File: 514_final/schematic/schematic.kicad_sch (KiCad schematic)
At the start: 21 parts, among them M1 Stepper_Motor_unipolar_5pin, SW1 SW_Push, SW2 SW_Push, U1 ULN2003

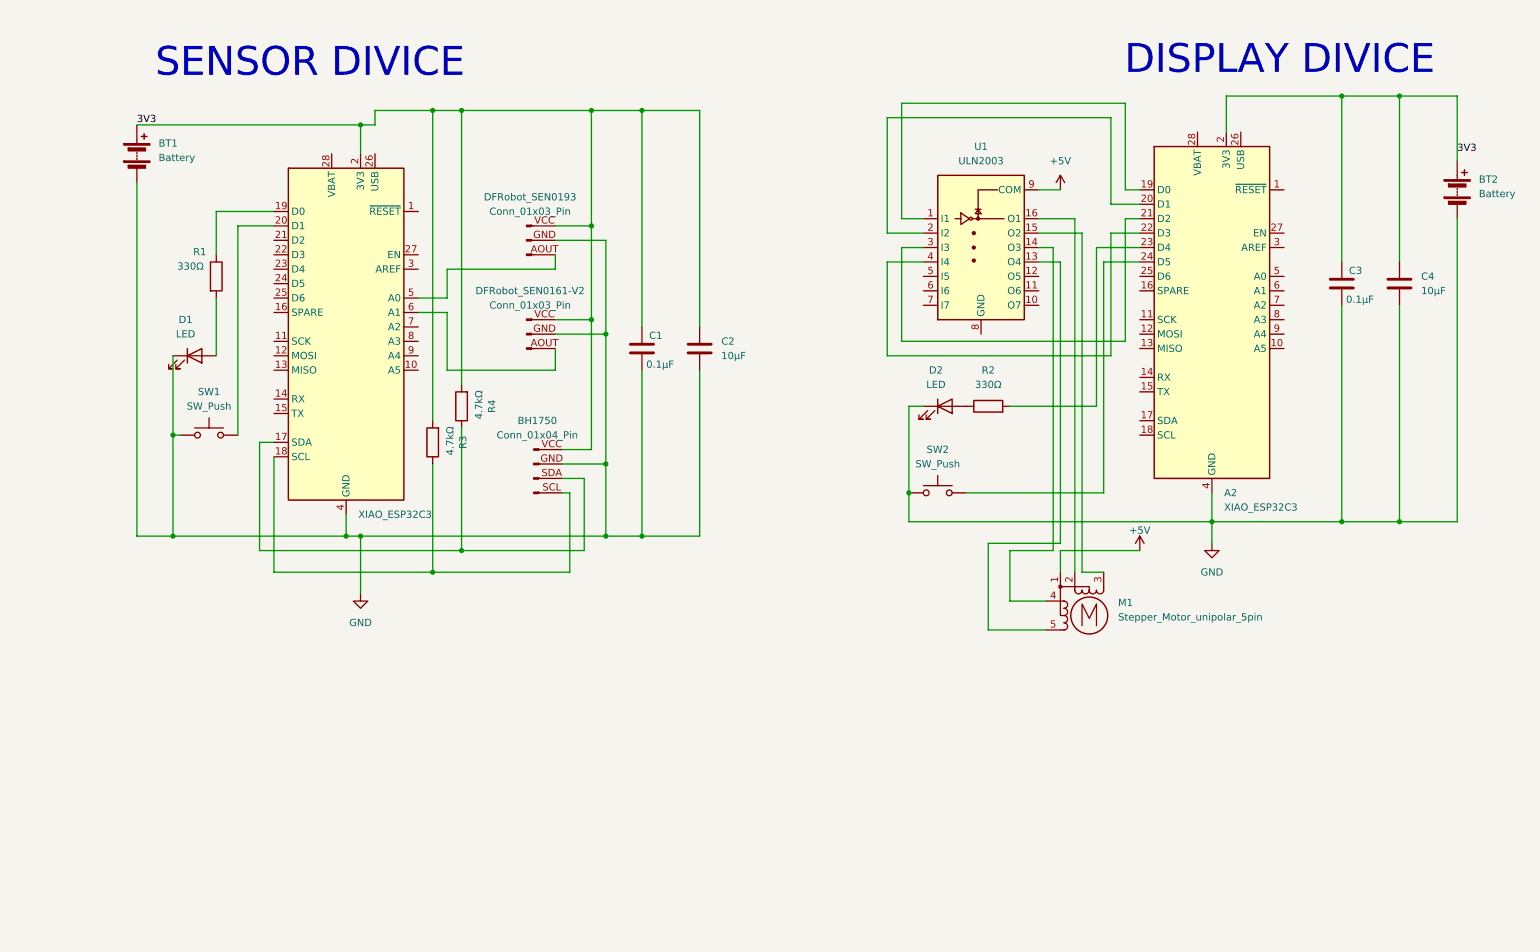
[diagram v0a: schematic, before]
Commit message: PCB 0203
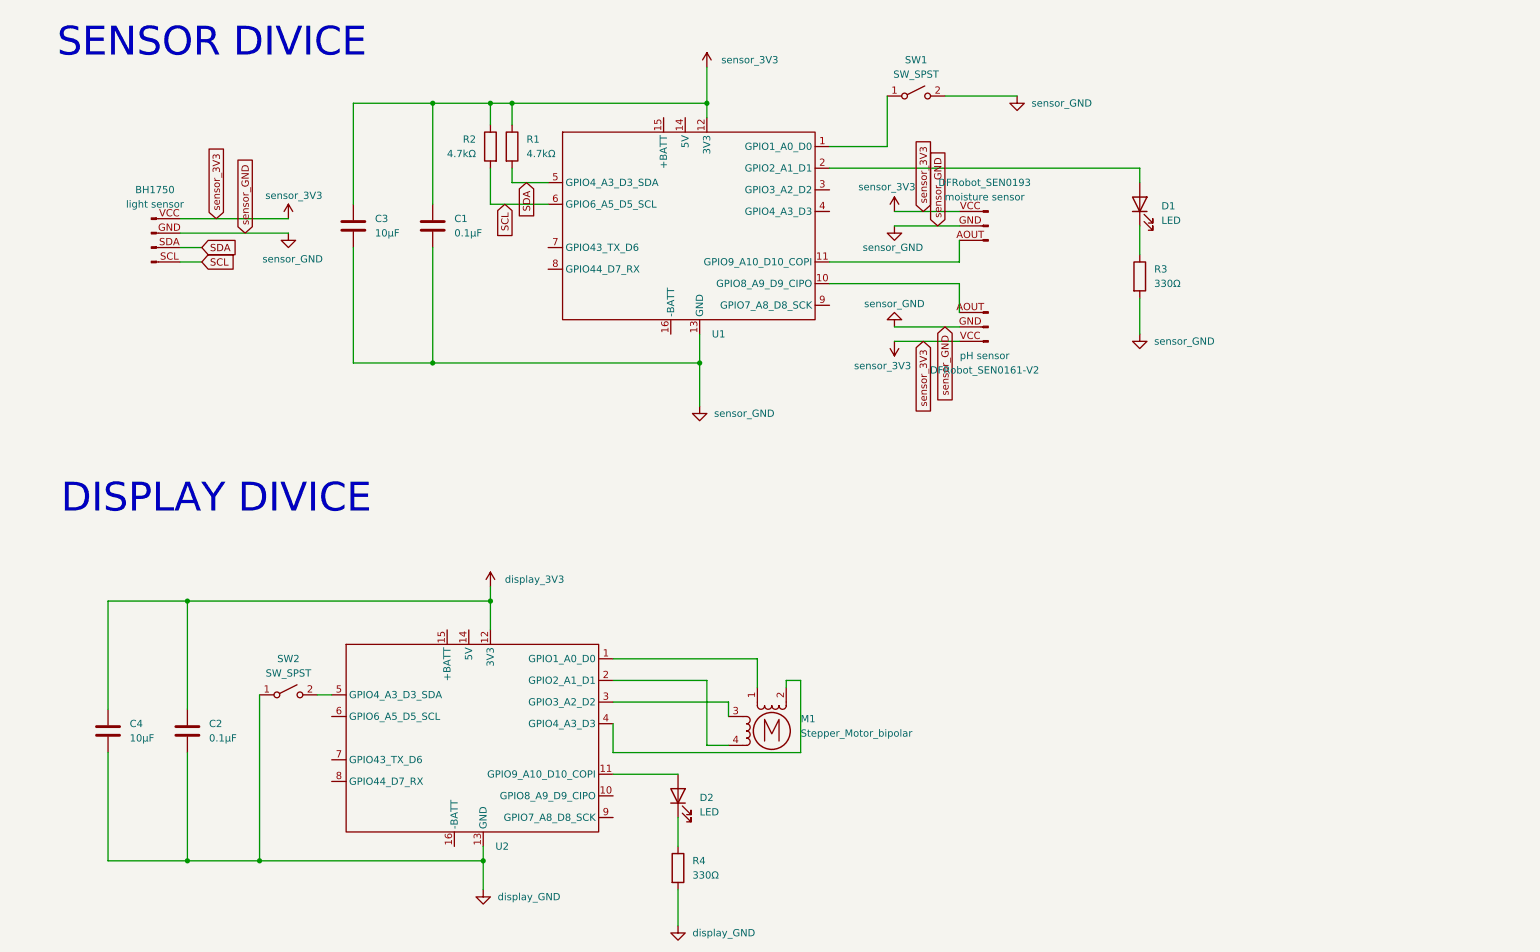
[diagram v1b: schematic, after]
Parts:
- removed A2: XIAO_ESP32C3, Module:Adafruit_Feather, symbol MCU_Module:Adafruit_Feather_Generic
- removed BT1, BT2: Battery, symbol Device:Battery
- removed M1: Stepper_Motor_unipolar_5pin, symbol Motor:Stepper_Motor_unipolar_5pin
- removed SW1, SW2: SW_Push, symbol Switch:SW_Push
- removed U1: ULN2003, symbol Transistor_Array:ULN2003
- removed XIAO_ESP32C3: Adafruit_Feather_Generic, Module:Adafruit_Feather, symbol MCU_Module:Adafruit_Feather_Generic
- added M1: Stepper_Motor_bipolar, 514final_Library:x27_stepper, symbol Motor:Stepper_Motor_bipolar
- added SW1, SW2: SW_SPST, Button_Switch_THT:SW_PUSH_6mm, symbol Switch:SW_SPST
- added U1, U2: ~, 514final_Library:XIAO_ESP32, symbol GIX_ESP32:XIAO_ESP32
- BH1750: value Conn_01x04_Pin -> light sensor; footprint (none) -> Connector_PinHeader_2.54mm:PinHeader_1x04_P2.54mm_Vertical
- C1, C4: footprint (none) -> Capacitor_SMD:C_0805_2012Metric
- C2: value 10μF -> 0.1μF; footprint (none) -> Capacitor_SMD:C_0805_2012Metric
- C3: value 0.1μF -> 10μF; footprint (none) -> Capacitor_SMD:C_0805_2012Metric
- D1, D2: footprint (none) -> LED_SMD:LED_0805_2012Metric
- DFRobot_SEN0161-V2: value Conn_01x03_Pin -> pH sensor; footprint (none) -> Connector_PinHeader_2.54mm:PinHeader_1x03_P2.54mm_Vertical
- DFRobot_SEN0193: value Conn_01x03_Pin -> moisture sensor; footprint (none) -> Connector_PinHeader_2.54mm:PinHeader_1x03_P2.54mm_Vertical
- R1, R2: value 330Ω -> 4.7kΩ; footprint (none) -> Capacitor_SMD:C_0805_2012Metric
- R3, R4: value 4.7kΩ -> 330Ω; footprint (none) -> Capacitor_SMD:C_0805_2012Metric
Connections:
- net at DFRobot_SEN0193.AOUT (Pin_3): now also U1.11 (GPIO9_A10_D10_COPI)
- net at D2.2 (A): now also U2.11 (GPIO9_A10_D10_COPI); no longer R2.1
- net at R3.1: now also D1.1 (K); no longer BH1750.SCL (Pin_4)
- net at D1.2 (A): now also U1.2 (GPIO2_A1_D1); no longer R1.2
- net at R4.1: now also D2.1 (K); no longer BH1750.SDA (Pin_3)
- net sensor_3V3: now reaches R1.1
- net sensor_3V3: now also BH1750.VCC (Pin_1), C1.1, C3.1, DFRobot_SEN0161-V2.VCC (Pin_1), DFRobot_SEN0193.VCC (Pin_1), R2.1, U1.12 (3V3)
- net at DFRobot_SEN0161-V2.AOUT (Pin_3): now also U1.10 (GPIO8_A9_D9_CIPO)
- net SCL: now reaches R2.2
- net SCL: now also BH1750.SCL (Pin_4), U1.6 (GPIO6_A5_D5_SCL)
- removed net 3V3: BH1750.VCC (Pin_1), C1.1, C2.1, C3.1, C4.1, DFRobot_SEN0161-V2.VCC (Pin_1), DFRobot_SEN0193.VCC (Pin_1), R3.2, R4.2
- net GND renamed sensor_GND
- net sensor_GND: now also R3.2, SW1.2 (B), U1.13 (GND); no longer C2.2, C4.2, D1.1 (K), D2.1 (K)
- new net: SW1.1 (A), U1.1 (GPIO1_A0_D0)
- new net: M1.1, U2.1 (GPIO1_A0_D0)
- new net: M1.2 (-), U2.4 (GPIO4_A3_D3)
- new net: M1.3, U2.3 (GPIO3_A2_D2)
- new net: M1.4, U2.2 (GPIO2_A1_D1)
- new net: SW2.2 (B), U2.5 (GPIO4_A3_D3_SDA)
- new net SDA: BH1750.SDA (Pin_3), R1.2, U1.5 (GPIO4_A3_D3_SDA)
- new net display_3V3: C2.1, C4.1, U2.12 (3V3)
- new net display_GND: C2.2, C4.2, R4.2, SW2.1 (A), U2.13 (GND)
